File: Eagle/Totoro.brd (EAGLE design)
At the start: 107.5 x 80.4 mm, 62 parts, among them IC1 MCP6004, J1 AUDIO_JACK_3.5MMDCI, T1 BC546A

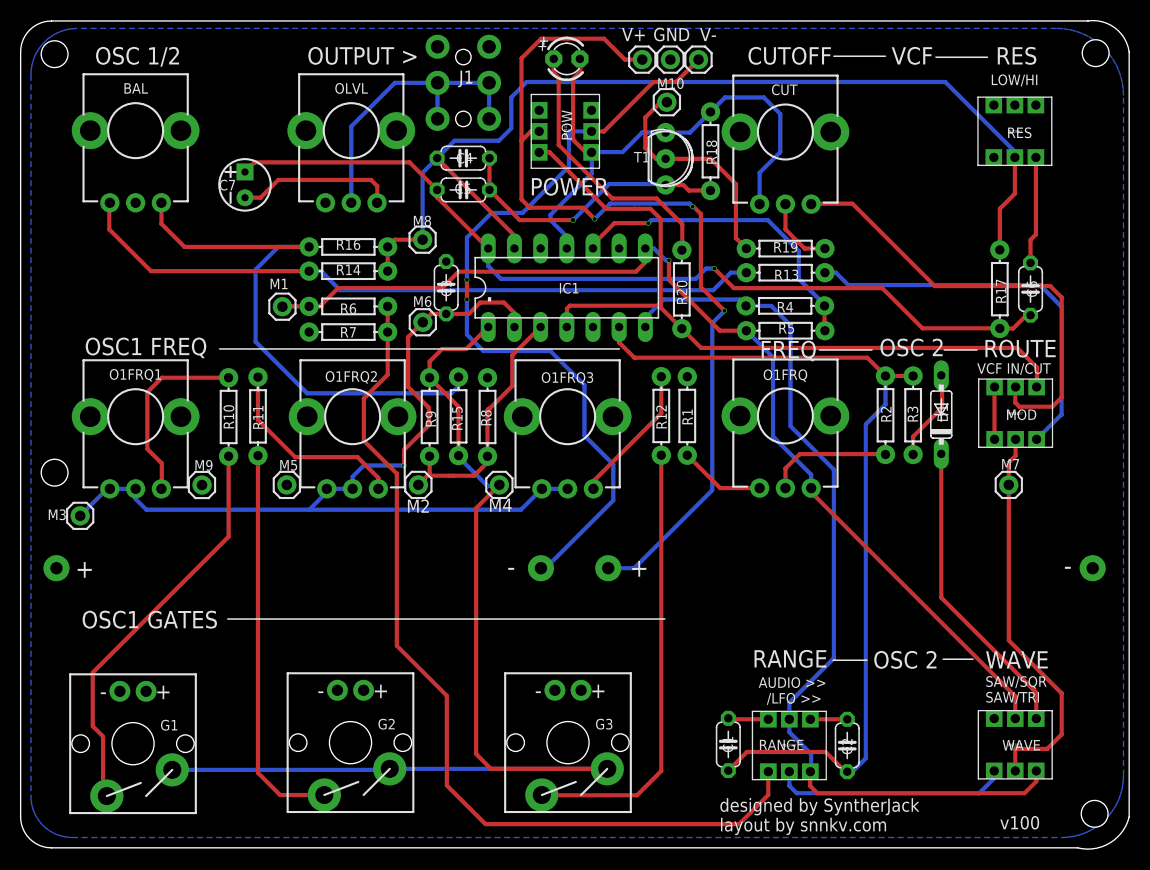
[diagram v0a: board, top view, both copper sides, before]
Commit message: version 101
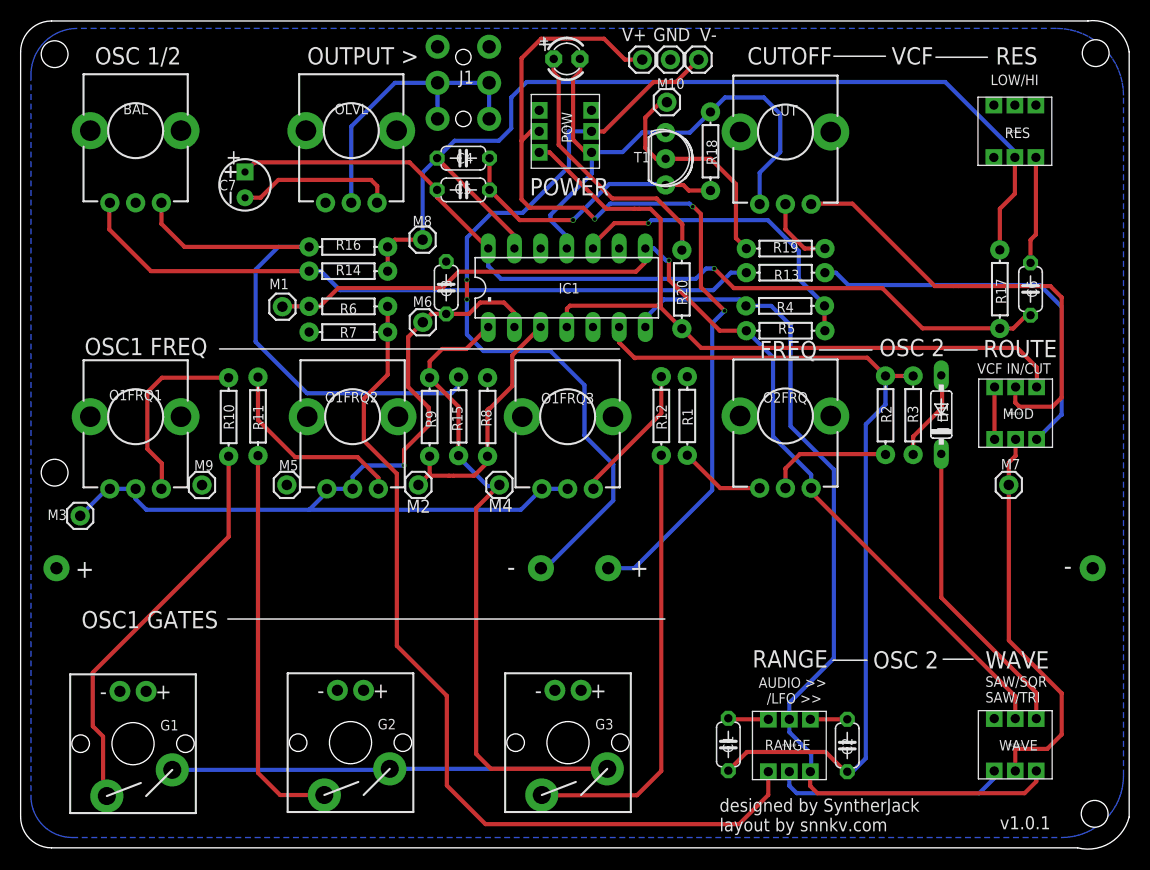
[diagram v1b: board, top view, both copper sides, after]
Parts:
- renumbered O1FRQ to O2FRQ
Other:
- board text added: "v1.0.1"
- board text removed: "v100"
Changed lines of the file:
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@@
 <text x="66.8" y="-3.4" size="1.27" layer="25" font="vector" ratio="10">designed by SyntherJack
 layout by snnkv.com</text>
-<text x="94" y="-3.2" size="1.27" layer="25" font="vector" ratio="10">v100</text>
+<text x="94" y="-3.2" size="1.27" layer="25" font="vector" ratio="10">v1.0.1</text>
 <rectangle x1="87.82003125" y1="47.265671875" x2="87.87336875" y2="47.283446875" layer="200"/>
 <rectangle x1="87.80225" y1="47.28345" x2="87.87336875" y2="47.30123125" layer="200"/>
@@
 <wire x1="60.2" y1="64.5" x2="60.2" y2="59.5" width="0.1524" layer="25"/>
 <wire x1="60.2" y1="64.5" x2="60.2" y2="59.5" width="0.1524" layer="25" curve="-223.602819"/>
-<text x="49.1" y="72.3" size="1.016" layer="25">+</text>
+<text x="49.1" y="72.3" size="1.5" layer="25">+</text>
+<wire x1="88" y1="35.6" x2="89" y2="35.6" width="0.25" layer="25"/>
+<text x="18.9" y="61.3" size="1.5" layer="25">+</text>
 </plain>
 <attributes>
@@
 <elements>
 <element name="BAL" library="SparkFun-Resistors" package="POT-PTH-ALPS-KIT" value="10k" x="10.16" y="64.58" smashed="yes" rot="R270">
-<attribute name="NAME" x="10.16" y="68.168" size="1.016" layer="25" ratio="10" align="bottom-center"/>
+<attribute name="NAME" x="10.16" y="66.168" size="1.016" layer="25" ratio="10" align="bottom-center"/>
 </element>
 <element name="C1" library="rcl" library_urn="urn:adsk.eagle:library:334" package="C050-024X044" package3d_urn="urn:adsk.eagle:package:23643/1" value="10n" x="67.66" y="5.03" smashed="yes" rot="R270">
@@
 </element>
 <element name="CUT" library="SparkFun-Resistors" package="POT-PTH-ALPS-KIT" value="10k" x="73.2" y="64.45" smashed="yes" rot="R270">
-<attribute name="NAME" x="73.1" y="68.038" size="1.016" layer="25" ratio="10" align="bottom-center"/>
+<attribute name="NAME" x="73.1" y="66.038" size="1.016" layer="25" ratio="10" align="bottom-center"/>
 </element>
 <element name="D1" library="diode" library_urn="urn:adsk.eagle:library:210" package="DO35-7" package3d_urn="urn:adsk.eagle:package:43339/2" value="1N4148DO35-7" x="88.32" y="37.03" smashed="yes" rot="R90">
@@
 <attribute name="VALUE" x="93.6" y="28.686" size="0.6096" layer="27" font="vector" ratio="20" align="top-left"/>
 </element>
-<element name="O1FRQ" library="SparkFun-Resistors" package="POT-PTH-ALPS-KIT" value="10k" x="73.2" y="36.9" smashed="yes" rot="R270">
-<attribute name="NAME" x="73.2" y="40.388" size="1.016" layer="25" ratio="10" align="bottom-center"/>
+<element name="O2FRQ" library="SparkFun-Resistors" package="POT-PTH-ALPS-KIT" value="10k" x="73.2" y="36.9" smashed="yes" rot="R270">
+<attribute name="NAME" x="73.2" y="38.188" size="1.016" layer="25" ratio="10" align="bottom-center"/>
 </element>
 <element name="O1FRQ1" library="SparkFun-Resistors" package="POT-PTH-ALPS-KIT" value="10k" x="10.16" y="36.83" smashed="yes" rot="R270">
-<attribute name="NAME" x="10.16" y="40.418" size="1.016" layer="25" ratio="10" align="bottom-center"/>
+<attribute name="NAME" x="10.16" y="38.418" size="1.016" layer="25" ratio="10" align="bottom-center"/>
 </element>
 <element name="O1FRQ2" library="SparkFun-Resistors" package="POT-PTH-ALPS-KIT" value="10k" x="31.21" y="36.83" smashed="yes" rot="R270">
-<attribute name="NAME" x="31.11" y="40.218" size="1.016" layer="25" ratio="10" align="bottom-center"/>
+<attribute name="NAME" x="31.11" y="38.218" size="1.016" layer="25" ratio="10" align="bottom-center"/>
 </element>
 <element name="O1FRQ3" library="SparkFun-Resistors" package="POT-PTH-ALPS-KIT" value="10k" x="52.07" y="36.83" smashed="yes" rot="R270">
-<attribute name="NAME" x="52.07" y="40.118" size="1.016" layer="25" ratio="10" align="bottom-center"/>
+<attribute name="NAME" x="52.07" y="38.118" size="1.016" layer="25" ratio="10" align="bottom-center"/>
 </element>
 <element name="OLVL" library="SparkFun-Resistors" package="POT-PTH-ALPS-KIT" value="10k" x="31.08" y="64.58" smashed="yes" rot="R270">
-<attribute name="NAME" x="31.08" y="68.168" size="1.016" layer="25" ratio="10" align="bottom-center"/>
+<attribute name="NAME" x="31.08" y="66.168" size="1.016" layer="25" ratio="10" align="bottom-center"/>
 </element>
 <element name="R1" library="SparkFun-Resistors" package="AXIAL-0.3" value="1k" x="63.68" y="36.9" smashed="yes" rot="R270">
@@
 </element>
 <element name="WAVE" library="atarity-switch-pb22e07" package="PB22E07" value="" x="97.5" y="7.5" smashed="yes" rot="R180">
-<attribute name="NAME" x="97.98" y="5.4598" size="1.016" layer="25" ratio="10" rot="R180"/>
+<attribute name="NAME" x="97.68" y="5.4598" size="1.016" layer="25" ratio="10" rot="R180"/>
 <attribute name="POPULARITY" value="2" x="58.13" y="51.95" size="1.778" layer="27" rot="R180" display="off"/>
 <attribute name="VALUE" x="101.945" y="10.675" size="1.27" layer="27" ratio="10" rot="R180"/>
 </element>
 <element name="RANGE" library="atarity-switch-pb22e07" package="PB22E07" value="" x="71.58" y="2.43" smashed="yes">
-<attribute name="NAME" x="70.6" y="4.4702" size="1.016" layer="25" ratio="10"/>
+<attribute name="NAME" x="71.2" y="4.4702" size="1.016" layer="25" ratio="10"/>
 <attribute name="POPULARITY" value="2" x="122.38" y="-42.02" size="1.778" layer="27" display="off"/>
 <attribute name="VALUE" x="67.135" y="-0.745" size="1.27" layer="27" ratio="10"/>
 </element>
 <element name="MOD" library="atarity-switch-pb22e07" package="PB22E07" value="" x="97.53" y="39.67" smashed="yes" rot="R180">
-<attribute name="NAME" x="97.61" y="37.5298" size="1.016" layer="25" ratio="10" rot="R180"/>
+<attribute name="NAME" x="97.31" y="37.6298" size="1.016" layer="25" ratio="10" rot="R180"/>
 <attribute name="POPULARITY" value="2" x="35.3" y="84.12" size="1.778" layer="27" rot="R180" display="off"/>
 <attribute name="VALUE" x="101.975" y="42.845" size="1.27" layer="27" ratio="10" rot="R180"/>
 </element>
 <element name="RES" library="atarity-switch-pb22e07" package="PB22E07" value="" x="97.46" y="67.02" smashed="yes" rot="R180">
-<attribute name="NAME" x="97.14" y="64.8798" size="1.016" layer="25" ratio="10" rot="R180"/>
+<attribute name="NAME" x="96.94" y="64.8798" size="1.016" layer="25" ratio="10" rot="R180"/>
 <attribute name="POPULARITY" value="2" x="23.8" y="111.47" size="1.778" layer="27" rot="R180" display="off"/>
 <attribute name="VALUE" x="101.905" y="70.195" size="1.27" layer="27" ratio="10" rot="R180"/>
@@
 </element>
 <element name="POW" library="atarity-switch-pb22e07" package="PB22E07" value="" x="49.35" y="66.51" smashed="yes" rot="R270">
-<attribute name="NAME" x="51.4902" y="66.59" size="1.016" layer="25" ratio="10" rot="R270"/>
+<attribute name="NAME" x="51.4902" y="66.39" size="1.016" layer="25" ratio="10" rot="R270"/>
 <attribute name="POPULARITY" value="2" x="49.35" y="66.51" size="1.778" layer="27" rot="R270" display="off"/>
 <attribute name="VALUE" x="46.175" y="70.955" size="1.27" layer="27" ratio="10" rot="R270"/>
@@
 <signals>
 <signal name="N$2">
-<contactref element="O1FRQ" pad="P$2"/>
+<contactref element="O2FRQ" pad="P$2"/>
 <contactref element="R2" pad="P$1"/>
 <wire x1="73.2" y1="29.9" x2="73.2" y2="31.8" width="0.4064" layer="1"/>
@@
 </signal>
 <signal name="N$3">
-<contactref element="O1FRQ" pad="P$1"/>
+<contactref element="O2FRQ" pad="P$1"/>
 <contactref element="R1" pad="P$2"/>
 <wire x1="66.87" y1="29.9" x2="70.7" y2="29.9" width="0.4064" layer="1"/>
@@
 <contactref element="R6" pad="P$2"/>
 <contactref element="R5" pad="P$1"/>
-<contactref element="O1FRQ" pad="P$3"/>
+<contactref element="O2FRQ" pad="P$3"/>
 <contactref element="WAVE" pad="2"/>
 <contactref element="IC1" pad="8"/>
